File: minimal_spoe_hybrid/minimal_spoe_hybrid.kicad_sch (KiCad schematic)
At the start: 14 parts, among them J1 TBP02R2-381-03BE, J3 CLP-103-02-G-D-BE

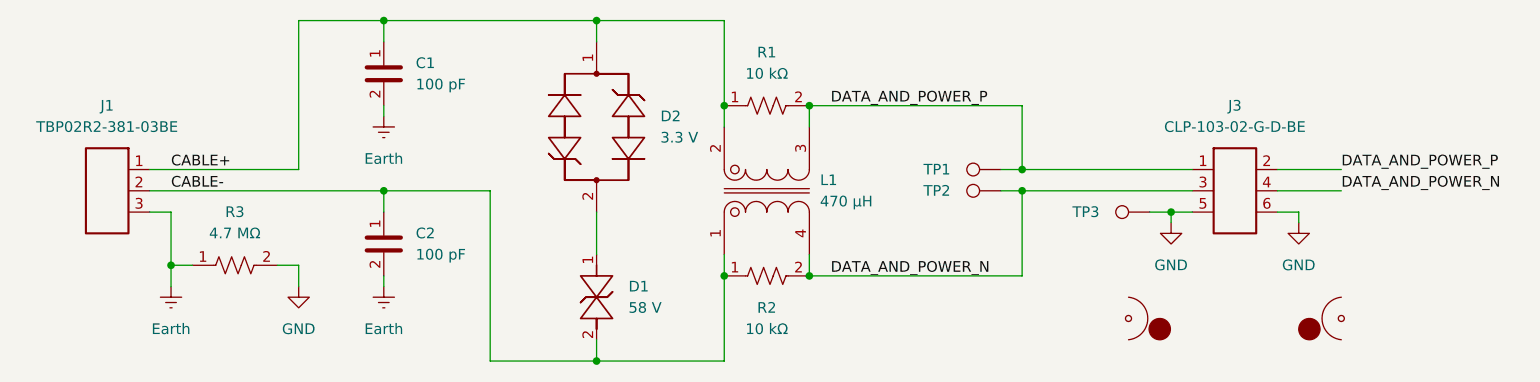
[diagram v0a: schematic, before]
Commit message: Switch to KiCad 9
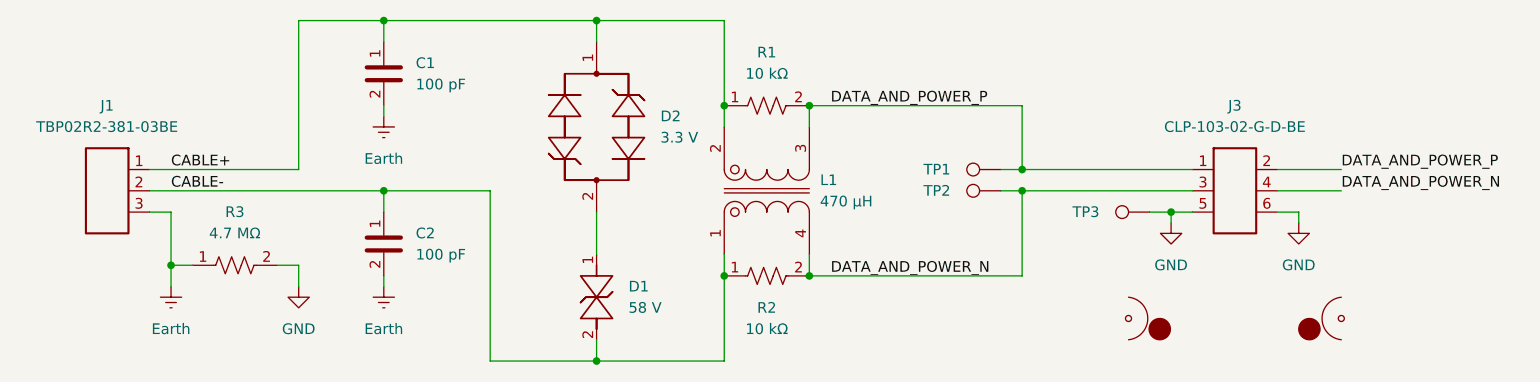
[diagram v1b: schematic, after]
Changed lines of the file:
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@@
 (kicad_sch
-	(version 20231120)
+	(version 20250114)
 	(generator "eeschema")
-	(generator_version "8.0")
+	(generator_version "9.0")
 	(paper "A4")
 	(junction
@@
 		)
 	)
+	(embedded_fonts no)
 )
